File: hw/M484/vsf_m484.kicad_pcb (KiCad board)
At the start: 4 copper layers, 34.9 x 30.5 mm, 82 parts, among them J1 Conn_02x10_Odd_Even, J2 USB_OTG, J3 USB_A, J4 USB_OTG, J5 Conn_01x05, J6 Conn_02x05_Odd_Even, U0 M4842U_64, U1 AP1117-33, U2 GD25Q_8P, U3 NUC120_64, U4 AP1117-33, Y0 Crystal_GND24, Y2 Crystal_GND24

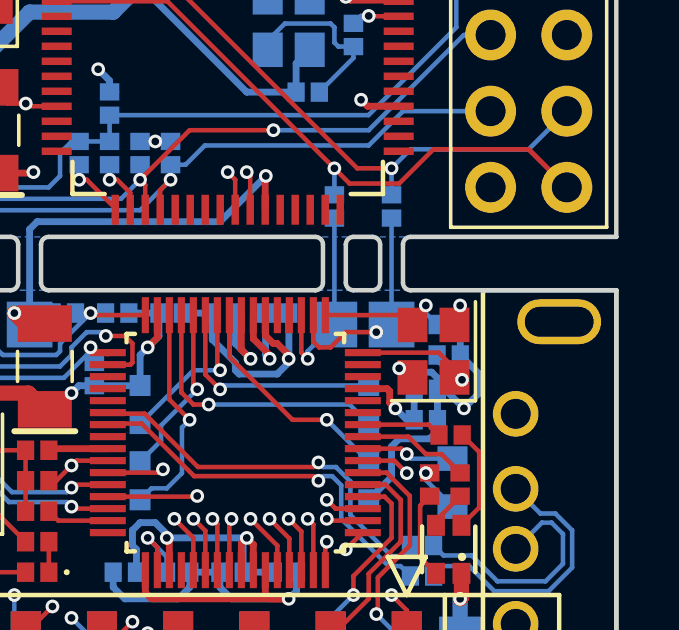
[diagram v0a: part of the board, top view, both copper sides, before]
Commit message: m484 pcb update
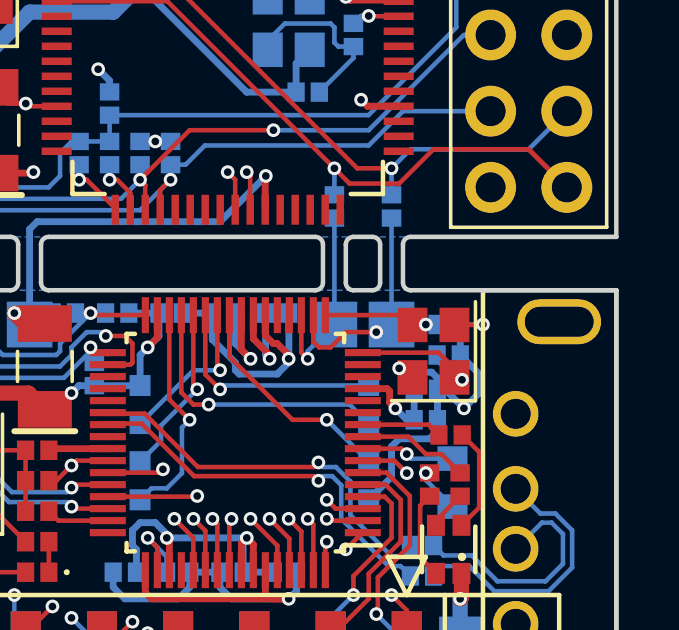
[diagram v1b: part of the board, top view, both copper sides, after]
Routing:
- net GND: track 253.3 -> 254.1 mm
- net /XT_OUT: track 4.66 -> 3.87 mm
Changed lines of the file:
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@@
     (thickness 1.6)
     (drawings 76)
-    (tracks 977)
+    (tracks 976)
     (zones 0)
     (modules 82)
@@
   (segment (start 201.724 110.03) (end 202.249 110.555) (width 0.1524) (layer F.Cu) (net 1))
   (segment (start 202.249 110.555) (end 202.249 110.857) (width 0.1524) (layer F.Cu) (net 1))
+  (segment (start 202.4445 109.093) (end 203.2 109.093) (width 0.1524) (layer B.Cu) (net 2))
+  (segment (start 203.186 109.107) (end 202.249 109.107) (width 0.1524) (layer F.Cu) (net 2))
+  (segment (start 203.2 109.093) (end 203.186 109.107) (width 0.1524) (layer F.Cu) (net 2))
+  (via (at 203.2 109.093) (size 0.4572) (drill 0.254) (layers F.Cu B.Cu) (net 2))
   (segment (start 202.249 109.107) (end 202.249 108.647) (width 0.2286) (layer F.Cu) (net 2))
-  (segment (start 202.249 108.647) (end 202.438 108.458) (width 0.2286) (layer F.Cu) (net 2))
-  (via (at 202.438 108.458) (size 0.4572) (drill 0.254) (layers F.Cu B.Cu) (net 2))
-  (segment (start 202.438 108.458) (end 202.4445 108.4645) (width 0.2286) (layer B.Cu) (net 2))
-  (segment (start 202.4445 108.4645) (end 202.4445 109.093) (width 0.2286) (layer B.Cu) (net 2))
   (segment (start 200.406 110.5535) (end 199.898 111.0615) (width 0.508) (layer In2.Cu) (net 2))
   (segment (start 199.898 111.0615) (end 196.723 111.0615) (width 0.508) (layer In2.Cu) (net 2))
@@
   (segment (start 190.8745 117.348) (end 190.8745 117.8495) (width 0.2286) (layer B.Cu) (net 2))
   (segment (start 190.8745 117.8495) (end 191.262 118.237) (width 0.2286) (layer B.Cu) (net 2))
-  (segment (start 200.849 109.107) (end 200.849 108.904) (width 0.1524) (layer F.Cu) (net 3))
-  (segment (start 200.849 108.904) (end 201.295 108.458) (width 0.1524) (layer F.Cu) (net 3))
-  (segment (start 201.295 108.7185) (end 201.6695 109.093) (width 0.1524) (layer B.Cu) (net 3))
-  (segment (start 201.295 108.458) (end 201.295 108.7185) (width 0.1524) (layer B.Cu) (net 3))
-  (via (at 201.295 108.458) (size 0.4572) (drill 0.254) (layers F.Cu B.Cu) (net 3))
+  (segment (start 200.849 109.107) (end 201.281 109.107) (width 0.1524) (layer F.Cu) (net 3))
+  (segment (start 201.281 109.107) (end 201.295 109.093) (width 0.1524) (layer F.Cu) (net 3))
+  (via (at 201.295 109.093) (size 0.4572) (drill 0.254) (layers F.Cu B.Cu) (net 3))
+  (segment (start 201.295 109.093) (end 201.6695 109.093) (width 0.1524) (layer B.Cu) (net 3))
   (segment (start 197.945 108.78) (end 200.522 108.78) (width 0.1524) (layer F.Cu) (net 3))
   (segment (start 200.522 108.78) (end 200.849 109.107) (width 0.1524) (layer F.Cu) (net 3))
